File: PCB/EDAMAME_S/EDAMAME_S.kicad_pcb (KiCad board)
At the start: 2 copper layers, 75 x 96 mm, 79 parts, among them CN1 USB-B-MICRO, J1 Conn, J2 ISP, J3 Conn, J4 Nichrome, J5 FlightPin, M1 Motor_L, M2 Motor_R, Q1 MTM231102LBF, Q2 2SC2712, SW1 power, U1 microSD, U10 LSM303C, U2 ATMEGA1284P-MU, U3 LSM303C, U4 TPS63001, U5 GYSFDMAXB, U6 FT231XQ, U7 BD6211F, U8 INA226, U9 BD6211F, Y1 16MHz

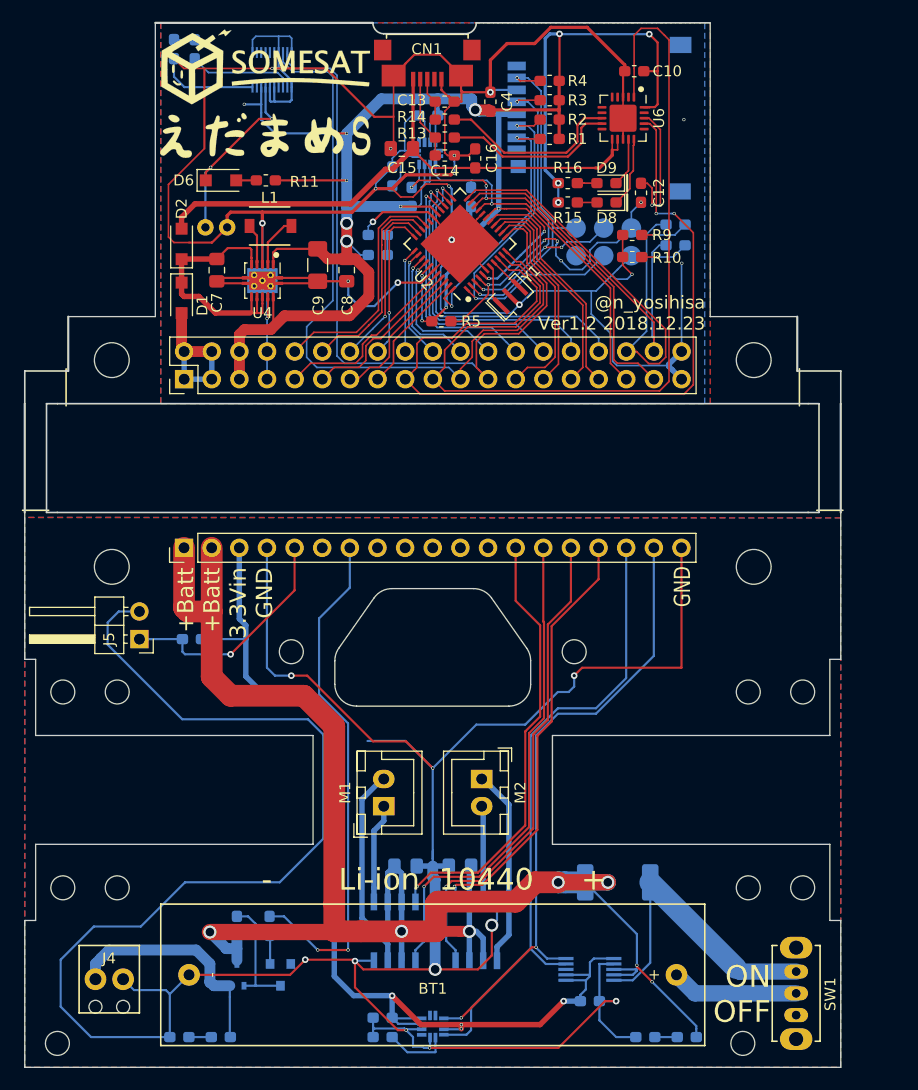
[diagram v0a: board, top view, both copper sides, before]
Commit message: EdamameS_V1.10
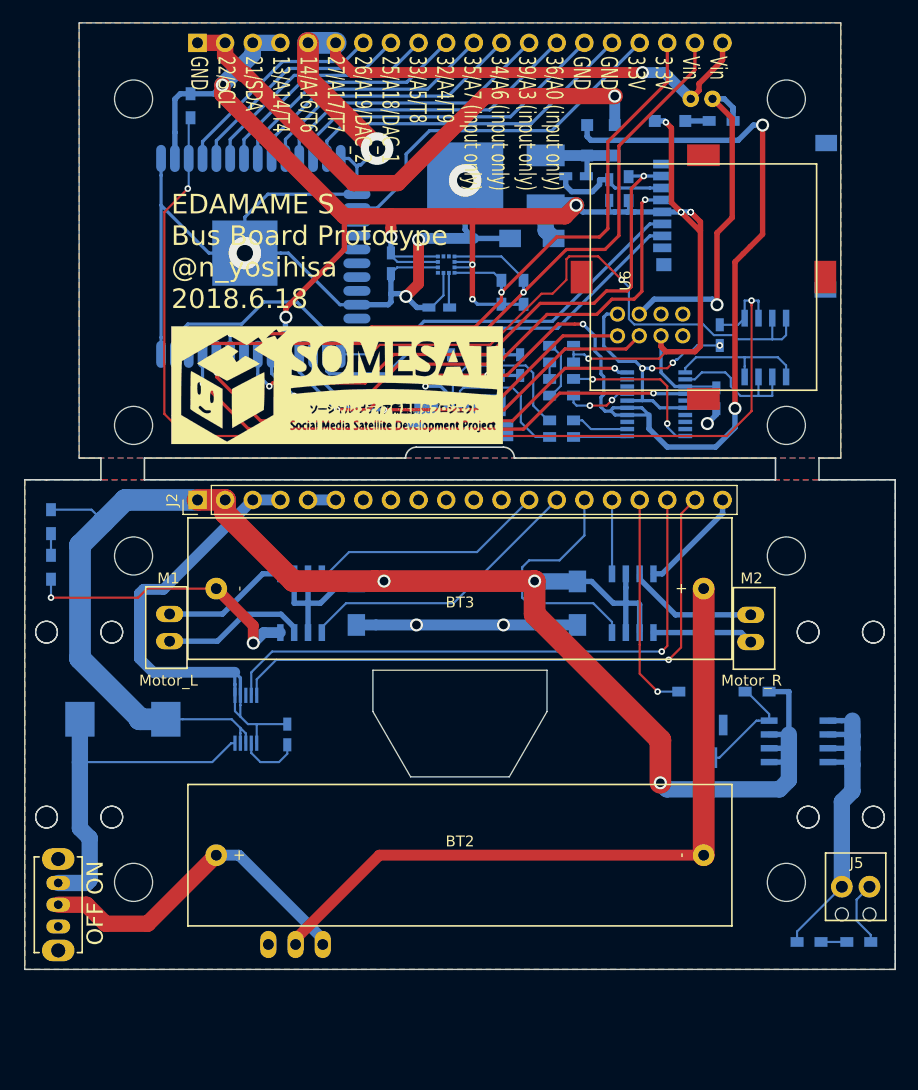
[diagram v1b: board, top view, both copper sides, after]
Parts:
- removed C15, C17, C19: 10u, Capacitor_SMD:C_0805_2012Metric_Pad1.15x1.40mm_HandSolder
- removed C16, C18, C20, C21: 0.1u, Capacitor_SMD:C_0603_1608Metric_Pad1.05x0.95mm_HandSolder
- removed D10: Nichrome, LED_SMD:LED_0603_1608Metric_Pad1.05x0.95mm_HandSolder
- removed D11: POWER, LED_SMD:LED_0603_1608Metric_Pad1.05x0.95mm_HandSolder
- removed D8: TX_LED, LED_SMD:LED_0603_1608Metric_Pad1.05x0.95mm_HandSolder
- removed D9: RX_LED, LED_SMD:LED_0603_1608Metric_Pad1.05x0.95mm_HandSolder
- removed the G*** at (50.6, 24.0)
- removed the G*** at (83.5, 70.6)
- removed J3: Conn, Connector_PinHeader_2.54mm:PinHeader_1x19_P2.54mm_Vertical
- removed J4: Nichrome, user:MPT0.5_2-2.54
- removed L1: 2.2uH, user:inductor_VLF4012-2R2
- removed R15, R16: 1k, Resistor_SMD:R_0603_1608Metric_Pad1.05x0.95mm_HandSolder
- removed R17, R19, R22: 10K, Resistor_SMD:R_0603_1608Metric_Pad1.05x0.95mm_HandSolder
- removed R18, R21: 1K, Resistor_SMD:R_0603_1608Metric_Pad1.05x0.95mm_HandSolder
- removed R20: 10m, Resistor_SMD:R_2512_6332Metric_Pad1.52x3.35mm_HandSolder
- removed U10: LSM303C, user:LGA-12_2x2mm_P0.5mm_HandSolder
- removed Y1: 16MHz, Crystal:Resonator_SMD_muRata_CSTxExxV-3Pin_3.0x1.1mm
- added BT2: 10440, user:BH-411, F.Cu at (68.6, 93.7)
- added BT3: 10440, user:BH-411, F.Cu at (68.6, 69.2)
- added C1: 0.1u, Capacitors_SMD:C_0603_HandSoldering, B.Cu at (92.1, 51.7)
- added G***: LOGO, mod:SOMESAT_LOGO, B.Cu at (74.5, 97.7)
- added G***: LOGO, mod:SOMESAT_LOGO, F.Cu at (57.3, 50.4)
- added J6: CHARGE, EH:S3B-EH, B.Cu at (53.4, 101.9)
- added Q3: 2SC2712, TO_SOT_Packages_SMD:SOT-23_Handsoldering, B.Cu at (91.8, 83.2)
- BT1: value 10440 -> BACKUP; footprint user:BH-411 -> user:MS621FE_FL11E; moved to B.Cu
- C10: value 0.1u -> 100u; footprint Capacitor_SMD:C_0603_1608Metric_Pad1.05x0.95mm_HandSolder -> Capacitors_SMD:C_1206_HandSoldering; moved to B.Cu
- C11: value 0.22F 3.3V -> 10u; footprint user:MS621FE_FL11E -> Capacitors_SMD:C_1206_HandSoldering
- C12: footprint Capacitor_SMD:C_0603_1608Metric_Pad1.05x0.95mm_HandSolder -> Capacitors_SMD:C_0603_HandSoldering; moved to B.Cu
- C13: value 47p -> 10u; footprint Capacitor_SMD:C_0603_1608Metric_Pad1.05x0.95mm_HandSolder -> Capacitors_SMD:C_1206_HandSoldering; moved to B.Cu
- C14: value 47p -> 10u; footprint Capacitor_SMD:C_0603_1608Metric_Pad1.05x0.95mm_HandSolder -> Capacitors_SMD:C_0603_HandSoldering; moved to B.Cu
- C2, C5: footprint Capacitor_SMD:C_0603_1608Metric_Pad1.05x0.95mm_HandSolder -> Capacitors_SMD:C_0603_HandSoldering
- C3: value 0.1u -> 47p; footprint Capacitor_SMD:C_0603_1608Metric_Pad1.05x0.95mm_HandSolder -> Capacitors_SMD:C_0603_HandSoldering
- C4: value 0.1u -> 47p; footprint Capacitor_SMD:C_0603_1608Metric_Pad1.05x0.95mm_HandSolder -> Capacitors_SMD:C_0603_HandSoldering; moved to B.Cu
- C6: value 0.1u -> 10u; footprint Capacitor_SMD:C_0603_1608Metric_Pad1.05x0.95mm_HandSolder -> Capacitors_SMD:C_0603_HandSoldering
- C7, C8: value 10u -> 0.1u; footprint Capacitor_SMD:C_0805_2012Metric_Pad1.15x1.40mm_HandSolder -> Capacitors_SMD:C_0603_HandSoldering; moved to B.Cu
- C9: value 100u -> 0.1u; footprint Capacitor_SMD:C_1206_3216Metric_Pad1.42x1.75mm_HandSolder -> Capacitors_SMD:C_0603_HandSoldering; moved to B.Cu
- CN1: footprint user:Micro-USB -> mylib:Micro-USB; moved to B.Cu
- D1: value GS1010FL -> TXLED; footprint Diode_SMD:D_SOD-123F -> LEDs:LED_0603_HandSoldering; moved to B.Cu
- D2: value GS1010FL -> RXLED; footprint Diode_SMD:D_SOD-123F -> LEDs:LED_0603_HandSoldering; moved to B.Cu
- D3: value POWER -> GS1010FL; footprint LED_SMD:LED_0603_1608Metric_Pad1.05x0.95mm_HandSolder -> Diodes_SMD:D_SOD-123F
- D4: value LED1 -> GS1010FL; footprint LED_SMD:LED_0603_1608Metric_Pad1.05x0.95mm_HandSolder -> Diodes_SMD:D_SOD-123F
- D5: value LED2 -> GS1010FL; footprint LED_SMD:LED_0603_1608Metric_Pad1.05x0.95mm_HandSolder -> Diodes_SMD:D_SOD-123F
- D6: value GS1010FL -> Nichrome; footprint Diode_SMD:D_SOD-123F -> LEDs:LED_0603_HandSoldering; moved to B.Cu
- D7: value 1PPS -> POWER; footprint LED_SMD:LED_0603_1608Metric_Pad1.05x0.95mm_HandSolder -> LEDs:LED_0603_HandSoldering
- J1: value Conn -> Conn_01x20; footprint Connector_PinHeader_2.54mm:PinHeader_2x19_P2.54mm_Vertical -> Socket_Strips:Socket_Strip_Straight_1x20_Pitch2.54mm; moved to B.Cu
- J2: value ISP -> Conn_01x20; footprint user:AVR_ISP -> Socket_Strips:Socket_Strip_Straight_1x20_Pitch2.54mm; moved to F.Cu
- J5: value FlightPin -> Nichrome; footprint Connector_PinHeader_2.54mm:PinHeader_1x02_P2.54mm_Horizontal -> user:MPT0.5_2-2.54
- M1, M2: footprint Connector_JST:JST_XH_B02B-XH-A_1x02_P2.50mm_Vertical -> EH:B2B-EH
- Q1: value MTM231102LBF -> NDS9936; footprint Package_TO_SOT_SMD:SOT-323_SC-70 -> Housings_SOIC:SOIC-8_3.9x4.9mm_Pitch1.27mm
- Q2: value 2SC2712 -> FDS4675; footprint Package_TO_SOT_SMD:SOT-23 -> Housings_SOIC:SOIC-8_3.9x4.9mm_Pitch1.27mm
- R1: value 10k -> 10K; footprint Resistor_SMD:R_0603_1608Metric_Pad1.05x0.95mm_HandSolder -> Resistors_SMD:R_0603_HandSoldering; moved to B.Cu
- R10: value 1k -> 1K; footprint Resistor_SMD:R_0603_1608Metric_Pad1.05x0.95mm_HandSolder -> Resistors_SMD:R_0603_HandSoldering; moved to B.Cu
- R11: value 100 -> 10K; footprint Resistor_SMD:R_0603_1608Metric_Pad1.05x0.95mm_HandSolder -> Resistors_SMD:R_0603_HandSoldering; moved to B.Cu
- R12: value 1k -> 10m; footprint Resistor_SMD:R_0603_1608Metric_Pad1.05x0.95mm_HandSolder -> Resistors_SMD:R_2512_HandSoldering
- R13: value 33 -> 1K; footprint Resistor_SMD:R_0603_1608Metric_Pad1.05x0.95mm_HandSolder -> Resistors_SMD:R_0603_HandSoldering; moved to B.Cu
- R14: value 33 -> 10K; footprint Resistor_SMD:R_0603_1608Metric_Pad1.05x0.95mm_HandSolder -> Resistors_SMD:R_0603_HandSoldering; moved to B.Cu
- R2, R3: value 10k -> 33; footprint Resistor_SMD:R_0603_1608Metric_Pad1.05x0.95mm_HandSolder -> Resistors_SMD:R_0603_HandSoldering; moved to B.Cu
- R4, R5: value 10k -> 1K; footprint Resistor_SMD:R_0603_1608Metric_Pad1.05x0.95mm_HandSolder -> Resistors_SMD:R_0603_HandSoldering; moved to B.Cu
- R6, R7: value 2.2k -> 2.2K; footprint Resistor_SMD:R_0603_1608Metric_Pad1.05x0.95mm_HandSolder -> Resistors_SMD:R_0603_HandSoldering
- R8: value 1k -> 100; footprint Resistor_SMD:R_0603_1608Metric_Pad1.05x0.95mm_HandSolder -> Resistors_SMD:R_0603_HandSoldering
- R9: value 1k -> 10K; footprint Resistor_SMD:R_0603_1608Metric_Pad1.05x0.95mm_HandSolder -> Resistors_SMD:R_0603_HandSoldering; moved to B.Cu
- SW1: footprint user:SS-12D01-VG4 -> mylib:SS-12D01-VG4
- U2: value ATMEGA1284P-MU -> FT231XS; footprint Package_DFN_QFN:QFN-44-1EP_7x7mm_P0.5mm_EP5.15x5.15mm -> SMD_Packages:SSOP-20; moved to B.Cu
- U3: value LSM303C -> ESP32-WROOM; footprint user:LGA-12_2x2mm_P0.5mm_HandSolder -> ESP32-footprints-Lib:ESP32-WROOM
- U4: value TPS63001 -> NJM2391DL1-33; footprint Package_SON:Texas_S-PVSON-N10_ThermalVias -> TO_SOT_Packages_SMD:TO-252-2_Rectifier; moved to B.Cu
- U5: value GYSFDMAXB -> LSM303C; footprint user:GYSFDMAXB -> Housings_LGA:LGA-12_2x2mm_Pitch0.5mm
- U6: value FT231XQ -> GPS-54D; footprint Package_DFN_QFN:QFN-20-1EP_4x4mm_P0.5mm_EP2.5x2.5mm -> user:GPS-54
- U7, U9: value BD6211F -> BD6231F; footprint Package_SO:SOIC-8_3.9x4.9mm_P1.27mm -> Housings_SOIC:SOIC-8_3.9x4.9mm_Pitch1.27mm
- U8: footprint Package_SO:MSOP-10_3x3mm_P0.5mm -> Housings_SSOP:MSOP-10_3x3mm_Pitch0.5mm
- moved D6 91.3 mm to (105.2, 101.6), turned to 180 degrees
- moved BT1 84.2 mm to (90.8, 24.1), turned to 180 degrees
- moved Q1 75.4 mm to (96.6, 47.0)
- moved SW1 68.3 mm to (31.6, 98.2)
- moved J5 68.2 mm to (102.2, 99.7), turned to 0 degrees
- moved R10 65.0 mm to (100.6, 101.6), turned to 0 degrees
- moved R12 61.9 mm to (37.6, 81.2), turned to 180 degrees
- moved R11 61.1 mm to (89.8, 78.6)
- moved C12 59.5 mm to (52.7, 82.6)
- moved Q2 52.2 mm to (99.7, 83.2), turned to 0 degrees
- moved R13 50.6 mm to (31.0, 63.0), turned to 270 degrees
- moved D7 48.9 mm to (31.0, 67.2)
- moved C11 47.9 mm to (79.4, 70.5), turned to 270 degrees
- moved C13 46.8 mm to (59.0, 70.5), turned to 270 degrees
- moved R9 43.5 mm to (95.9, 78.6), turned to 0 degrees
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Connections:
- BT1 pad 2: GNDPWR -> GND
- C11 pad 1: Net-(C11-Pad1) -> +BATT
- C11 pad 2: GND -> GNDPWR
- C12 pad 1: Net-(C12-Pad1) -> VCC
- C12 pad 2: /EDAMAME_S_core/RST -> GNDPWR
- C13 pad 1: Net-(C13-Pad1) -> +BATT
- C13 pad 2: GND -> GNDPWR
- C14 pad 1: Net-(C14-Pad1) -> /EN
- C3 pad 1: +3V3 -> Net-(C3-Pad1)
- C4 pad 1: +3V3 -> Net-(C4-Pad1)
- C5 pad 1: +3V3 -> +5V
- C6 pad 1: Net-(C6-Pad1) -> +5V
- C7 pad 1: Net-(C7-Pad1) -> +3V3
- C8 pad 1: +3V3 -> Net-(C8-Pad1)
- C9 pad 1: +3V3 -> Net-(C9-Pad1)
- CN1 pad 2: Net-(C14-Pad1) -> Net-(C4-Pad1)
- CN1 pad 3: Net-(C13-Pad1) -> Net-(C3-Pad1)
- D1 pad 1: Net-(C7-Pad1) -> Net-(D1-Pad1)
- D2 pad 1: Net-(C7-Pad1) -> Net-(D2-Pad1)
- D2 pad 2: +5V -> Net-(D2-Pad2)
- D3 pad 1: GND -> Net-(C9-Pad1)
- D3 pad 2: Net-(D3-Pad2) -> +5V
- D4 pad 1: Net-(D4-Pad1) -> Net-(C9-Pad1)
- D4 pad 2: /EDAMAME_S_core/19 -> VDC
- D5 pad 2: /EDAMAME_S_core/18 -> +3V3
- D6 pad 1: Net-(C11-Pad1) -> GNDPWR
- D7 pad 1: GND -> GNDPWR
- J1 pad 1: Net-(D1-Pad2) -> VDC
- J1 pad 10: /EDAMAME_S_core/A7 -> /IO35
- J1 pad 11: /EDAMAME_S_core/1 -> /IO32
- J1 pad 12: /EDAMAME_S_core/A6 -> /IO33
- J1 pad 13: /EDAMAME_S_core/2 -> /IO25
- J1 pad 14: /EDAMAME_S_core/A5 -> /IO26
- J1 pad 15: /EDAMAME_S_core/3- -> /IO27
- J1 pad 16: /EDAMAME_S_core/A4 -> /IO14
- J1 pad 17: /EDAMAME_S_core/PC→AVR -> /IO13
- J1 pad 18: /EDAMAME_S_core/A3 -> /I2C_SDA
- J1 pad 19: /EDAMAME_S_core/AVR→PC -> /I2C_SCL
- J1 pad 2: Net-(D1-Pad2) -> VDC
- J1 pad 20: /EDAMAME_S_core/A2 -> GND
- J1 pad 3: Net-(D1-Pad2) -> +3V3
- J1 pad 4: Net-(D1-Pad2) -> +3V3
- J1 pad 5: +3V3 -> GND
- J1 pad 6: +3V3 -> GND
- J1 pad 7: GND -> /S_VP
- J1 pad 8: GND -> /S_VN
- J1 pad 9: /EDAMAME_S_core/0 -> /IO34
- J2 pad 1: /EDAMAME_S_core/MISO -> +BATT
- J2 pad 2: (no net) -> +BATT
- J2 pad 3: /EDAMAME_S_core/SCK -> VCC
- J2 pad 4: /EDAMAME_S_core/MOSI -> VCC
- J2 pad 5: /EDAMAME_S_core/RST -> GNDPWR
- J2 pad 6: GND -> GNDPWR
- J5 pad 1: /EDAMAME_S_Ex/FlightPin -> Net-(J5-Pad1)
- Q1 pad 1: Net-(Q1-Pad1) -> /DTR
- Q1 pad 2: Net-(J4-Pad1) -> /RST
- Q1 pad 3: +BATT -> /RST
- Q2 pad 1: Net-(Q2-Pad1) -> +BATT
- Q2 pad 2: GNDPWR -> +BATT
- Q2 pad 3: Net-(Q1-Pad1) -> +BATT
- R1 pad 1: /EDAMAME_S_core/SS -> +3V3
- R1 pad 2: +3V3 -> /SPI_MISO
- R10 pad 1: Net-(D5-Pad1) -> Net-(J5-Pad1)
- R10 pad 2: GND -> Net-(D6-Pad2)
- R11 pad 1: +3V3 -> Net-(Q3-Pad1)
- R11 pad 2: Net-(D6-Pad2) -> /Nichrome
- R12 pad 1: Net-(D7-Pad2) -> +BATT
- R13 pad 1: Net-(R13-Pad1) -> +BATT
- R13 pad 2: Net-(C14-Pad1) -> Net-(D7-Pad2)
- R14 pad 1: Net-(R14-Pad1) -> /EN
- R14 pad 2: Net-(C13-Pad1) -> +3V3
- R2 pad 1: /EDAMAME_S_core/MOSI -> Net-(R2-Pad1)
- R2 pad 2: +3V3 -> Net-(C4-Pad1)
- R3 pad 1: /EDAMAME_S_core/SCK -> Net-(R3-Pad1)
- R3 pad 2: +3V3 -> Net-(C3-Pad1)
- R4 pad 1: /EDAMAME_S_core/MISO -> +3V3
- R4 pad 2: +3V3 -> Net-(D1-Pad2)
- R5 pad 2: /EDAMAME_S_core/RST -> Net-(D2-Pad2)
- R6 pad 1: +3V3 -> /I2C_SDA
- R6 pad 2: /EDAMAME_S_core/I2C_SDA -> +3V3
- R7 pad 1: +3V3 -> /I2C_SCL
- R7 pad 2: /EDAMAME_S_core/I2C_SCL -> +3V3
- R8 pad 1: Net-(D3-Pad2) -> Net-(BT1-Pad1)
- R8 pad 2: +3V3 -> Net-(D5-Pad1)
- R9 pad 1: Net-(D4-Pad1) -> Net-(Q2-Pad4)
- R9 pad 2: GND -> +BATT
- SW1 pad 1: Net-(R20-Pad2) -> Net-(R12-Pad2)
- SW1 pad 2: Net-(BT1-Pad1) -> Net-(BT2-Pad1)
- U1 pad 2: /EDAMAME_S_core/SS -> /SPI_CS
- U1 pad 3: /EDAMAME_S_core/MOSI -> /SPI_MOSI
- U1 pad 5: /EDAMAME_S_core/SCK -> /SPI_SCLK
- U1 pad 7: /EDAMAME_S_core/MISO -> /SPI_MISO
- U2 pad 1: /EDAMAME_S_core/MOSI -> /DTR
- U2 pad 10: /EDAMAME_S_core/AVR→PC -> Net-(D2-Pad1)
- U2 pad 11: /EDAMAME_S_core/GPS→AVR -> Net-(R3-Pad1)
- U2 pad 12: /EDAMAME_S_core/AVR→GPS -> Net-(R2-Pad1)
- U2 pad 13: /EDAMAME_S_core/12- -> (no net)
- U2 pad 14: /EDAMAME_S_core/13- -> +5V
- U2 pad 15: /EDAMAME_S_core/14- -> +5V
- U2 pad 16: /EDAMAME_S_core/15- -> GND
- U2 pad 17: +3V3 -> Net-(D1-Pad1)
- U2 pad 18: GND -> (no net)
- U2 pad 19: /EDAMAME_S_core/I2C_SCL -> (no net)
- U2 pad 2: /EDAMAME_S_core/MISO -> /RST
- U2 pad 20: /EDAMAME_S_core/I2C_SDA -> /PC→ESP32
- U2 pad 3: /EDAMAME_S_core/SCK -> +3V3
- U2 pad 4: /EDAMAME_S_core/RST -> /ESP32→PC
- U2 pad 5: +3V3 -> (no net)
- U2 pad 7: Net-(U2-Pad7) -> (no net)
- U2 pad 8: Net-(U2-Pad8) -> (no net)
- U2 pad 9: /EDAMAME_S_core/PC→AVR -> (no net)
- U3 pad 1: /EDAMAME_S_core/I2C_SCL -> GND
- U3 pad 10: +3V3 -> /IO25
- U3 pad 11: (no net) -> /IO26
- U3 pad 12: (no net) -> /IO27
- U3 pad 3: +3V3 -> /EN
- U3 pad 4: /EDAMAME_S_core/I2C_SDA -> /S_VP
- U3 pad 5: Net-(C6-Pad1) -> /S_VN
- U3 pad 6: GND -> /IO34
- U3 pad 7: (no net) -> /IO35
- U3 pad 8: GND -> /IO32
- U3 pad 9: +3V3 -> /IO33
- U4 pad 1: +3V3 -> Net-(C9-Pad1)
- U4 pad 2: Net-(L1-Pad2) -> GND
- U4 pad 3: GND -> +3V3
- U5 pad 1: GND -> /I2C_SCL
- U5 pad 10: GND -> +3V3
- U5 pad 12: GND -> (no net)
- U5 pad 2: GND -> +3V3
- U5 pad 3: /EDAMAME_S_core/AVR→GPS -> +3V3
- U5 pad 4: (no net) -> /I2C_SDA
- U5 pad 5: /EDAMAME_S_core/GPS→AVR -> Net-(C8-Pad1)
- U5 pad 6: Net-(R12-Pad2) -> GND
- U5 pad 7: GND -> (no net)
- U5 pad 8: (no net) -> GND
- U5 pad 9: (no net) -> +3V3
- U6 pad 1: /EDAMAME_S_core/AVR→PC -> /ESP32→GPS
- U6 pad 2: (no net) -> GND
- U6 pad 3: GND -> /GPS→ESP32
- U6 pad 4: (no net) -> Net-(BT1-Pad1)
- U6 pad 5: (no net) -> +3V3
- U6 pad 8: Net-(R14-Pad1) -> (no net)
- U7 pad 4: /EDAMAME_S_Ex/MOTOR_LF -> /MOTOR_LF
- U7 pad 5: /EDAMAME_S_Ex/MOTOR_LR -> /MOTOR_LR
- U8 pad 10: Net-(R20-Pad2) -> Net-(R12-Pad2)
- U8 pad 4: /EDAMAME_S_Ex/SDA -> /SDA
- U8 pad 5: /EDAMAME_S_Ex/SCL -> /SCL
- U9 pad 4: /EDAMAME_S_Ex/MOTOR_RR -> /MOTOR_RR
- U9 pad 5: /EDAMAME_S_Ex/MOTOR_RF -> /MOTOR_RF
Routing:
- net GNDPWR: track 278.2 -> 71.1 mm, vias 10 -> 4
- net /EN: track 0.00 -> 101.2 mm, vias 0 -> 2
- net GND: track 313.1 -> 212.6 mm, vias 18 -> 11
- net /EDAMAME_S_core/AVR→PC: track 83.5 -> 0.00 mm
- net /EDAMAME_S_core/PC→AVR: track 76.8 -> 0.00 mm, vias 2 -> 0
- net /I2C_SCL: track 0.00 -> 74.9 mm, vias 0 -> 2
- net /EDAMAME_S_core/AVR→GPS: track 68.1 -> 0.00 mm
- net /EDAMAME_S_core/GPS→AVR: track 66.2 -> 0.00 mm
- net /I2C_SDA: track 0.00 -> 66.1 mm, vias 0 -> 2
- net Net-(BT2-Pad2): track 0.00 -> 65.7 mm
- net /EDAMAME_S_Ex/SDA: track 58.9 -> 0.00 mm
- net /EDAMAME_S_Ex/SCL: track 57.7 -> 0.00 mm, vias 2 -> 0
- net /SCL: track 0.00 -> 55.8 mm, vias 0 -> 1
- net /SDA: track 0.00 -> 54.8 mm, vias 0 -> 1
- net /BOOT: track 0.00 -> 54.3 mm, vias 0 -> 2
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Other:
- board size 75 x 96 mm -> 80 x 87 mm
- rule via_min_drill: 0.2 -> 0.3
- rule via_min_size: 0.3 -> 0.6048
- board text added: "+ -"
- board text added: "@n_yosihisa 2018.6.18 EDAMAME S Extension Board"
- board text added: "EDAMAME S Bus Board Prototype @n_yosihisa 2018.6.18"
- board text added: "OFF ON"
- board text added: "Vin Vin 3.3V 3.3V GND GND 36/A0 (input only) 39/A3 (input only) 34/A6 (input only) 35/A7 (input only) 32/A4/T9 33/A5/T8 25/A18/DAC_1 26/A19/DAC_2 27/A17/T7 14/A16/T6 13/A14/T4 21/SDA 22/SCL GND"
- board text removed: "+Batt +Batt 3.3Vin GND"
- board text removed: "- Li-ion 10440 +"
- board text removed: "@n_yosihisa Ver1.2 2018.12.23"
- board text removed: "EDAMAME S @n_yosihisa Ver1.2 2018.12.23"
- board text removed: "GND"
- board text removed: "ISP"
- board text removed: "ON OFF"
- board text removed: "Vin Vin 3.3V GND"
